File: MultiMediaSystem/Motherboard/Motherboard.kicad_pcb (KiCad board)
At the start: 4 copper layers, 172.8 x 157.7 mm, 43 parts, among them J1 Wire Harness, J10 RF_EN, J14 5V_1, J15 RPI_Buck, J16 AUSB2-4599, J17 Illum/Dim, J18 5V_2, J19 GP_Buck, J2 Vmem Jumper, J20 5V_3, J21 Motherboard bracket, J22 Motherboard bracket, J3 Vacc_jumper, J4 RF_RX, J5 RF_CTRL, J6 AntennaExternal, J7 PwrCtrl_in, J8 RF_TX, J9 AntennaPwr_Conn, K1 ADW1112HTW, Q1 T2N7002BK,LM, U1 AudioAmp_PS, U2 AudioAmp, U3 PowerSupplyCtrl, U4 RadioRegulator, U5 HMC784AMS8GETR, U6 RadioAmp, U7 SN74LVC2G06QDCKRQ1

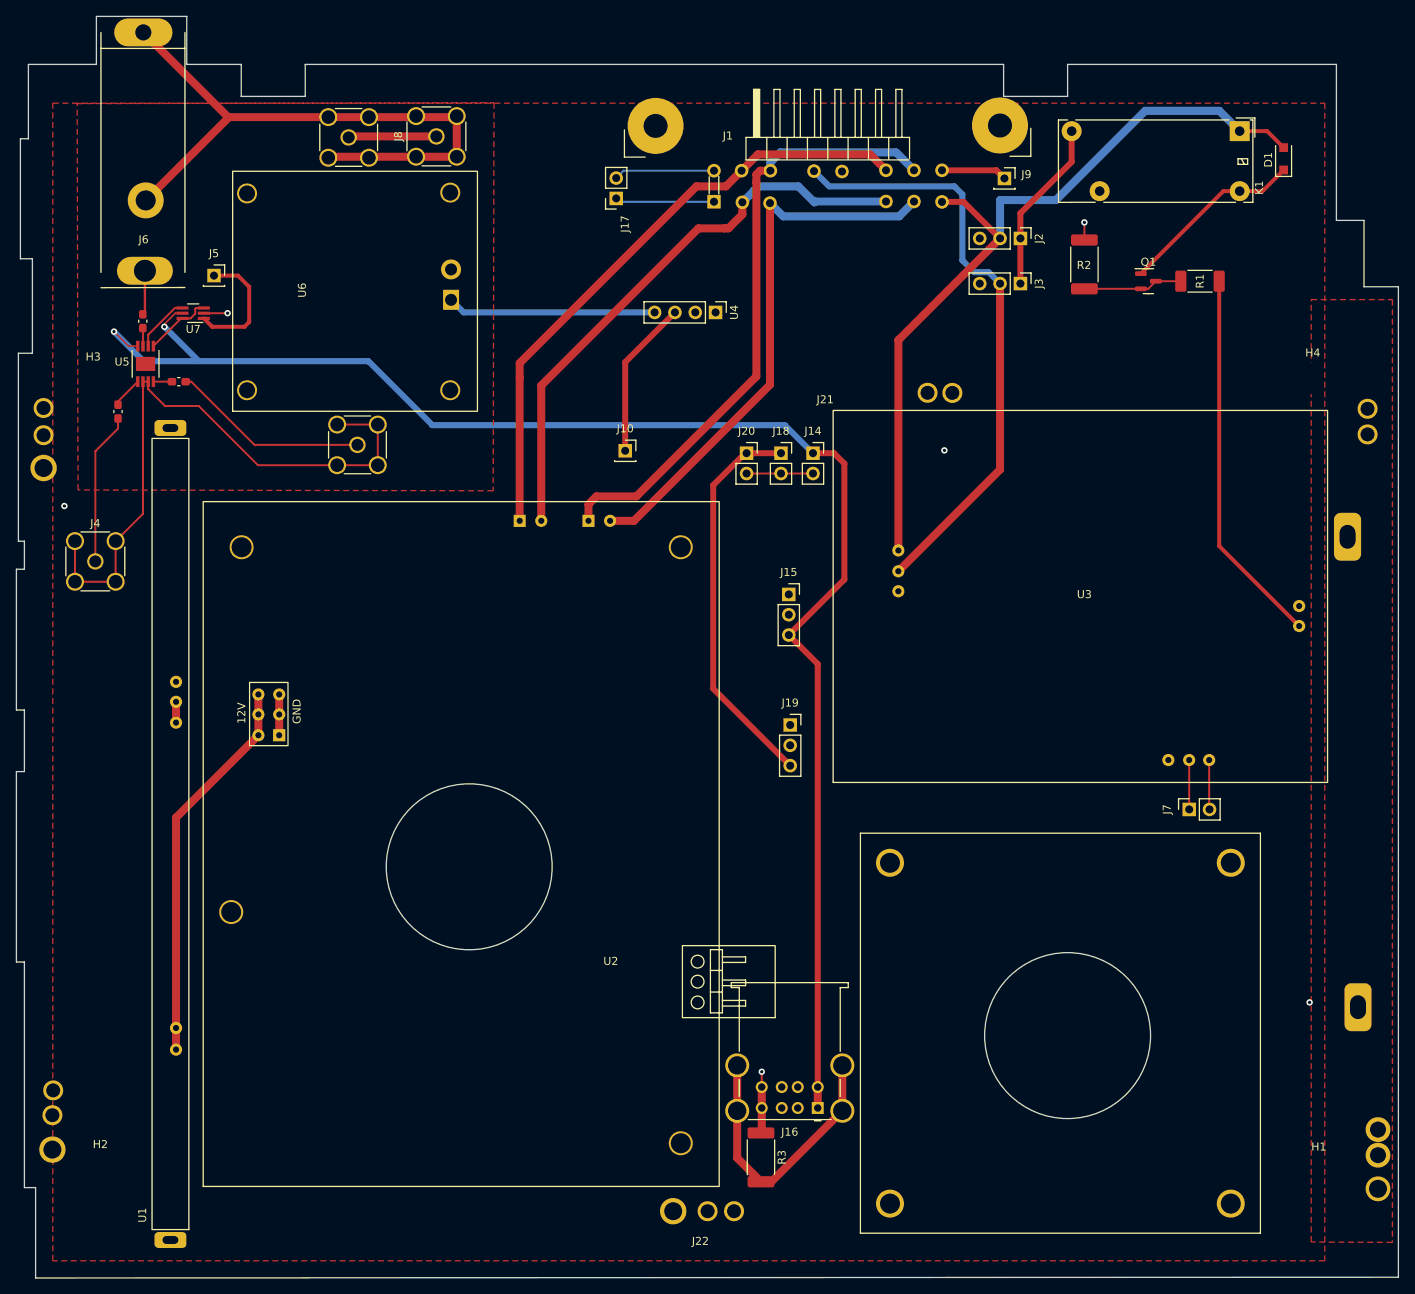
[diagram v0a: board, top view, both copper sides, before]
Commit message: Updated all designs
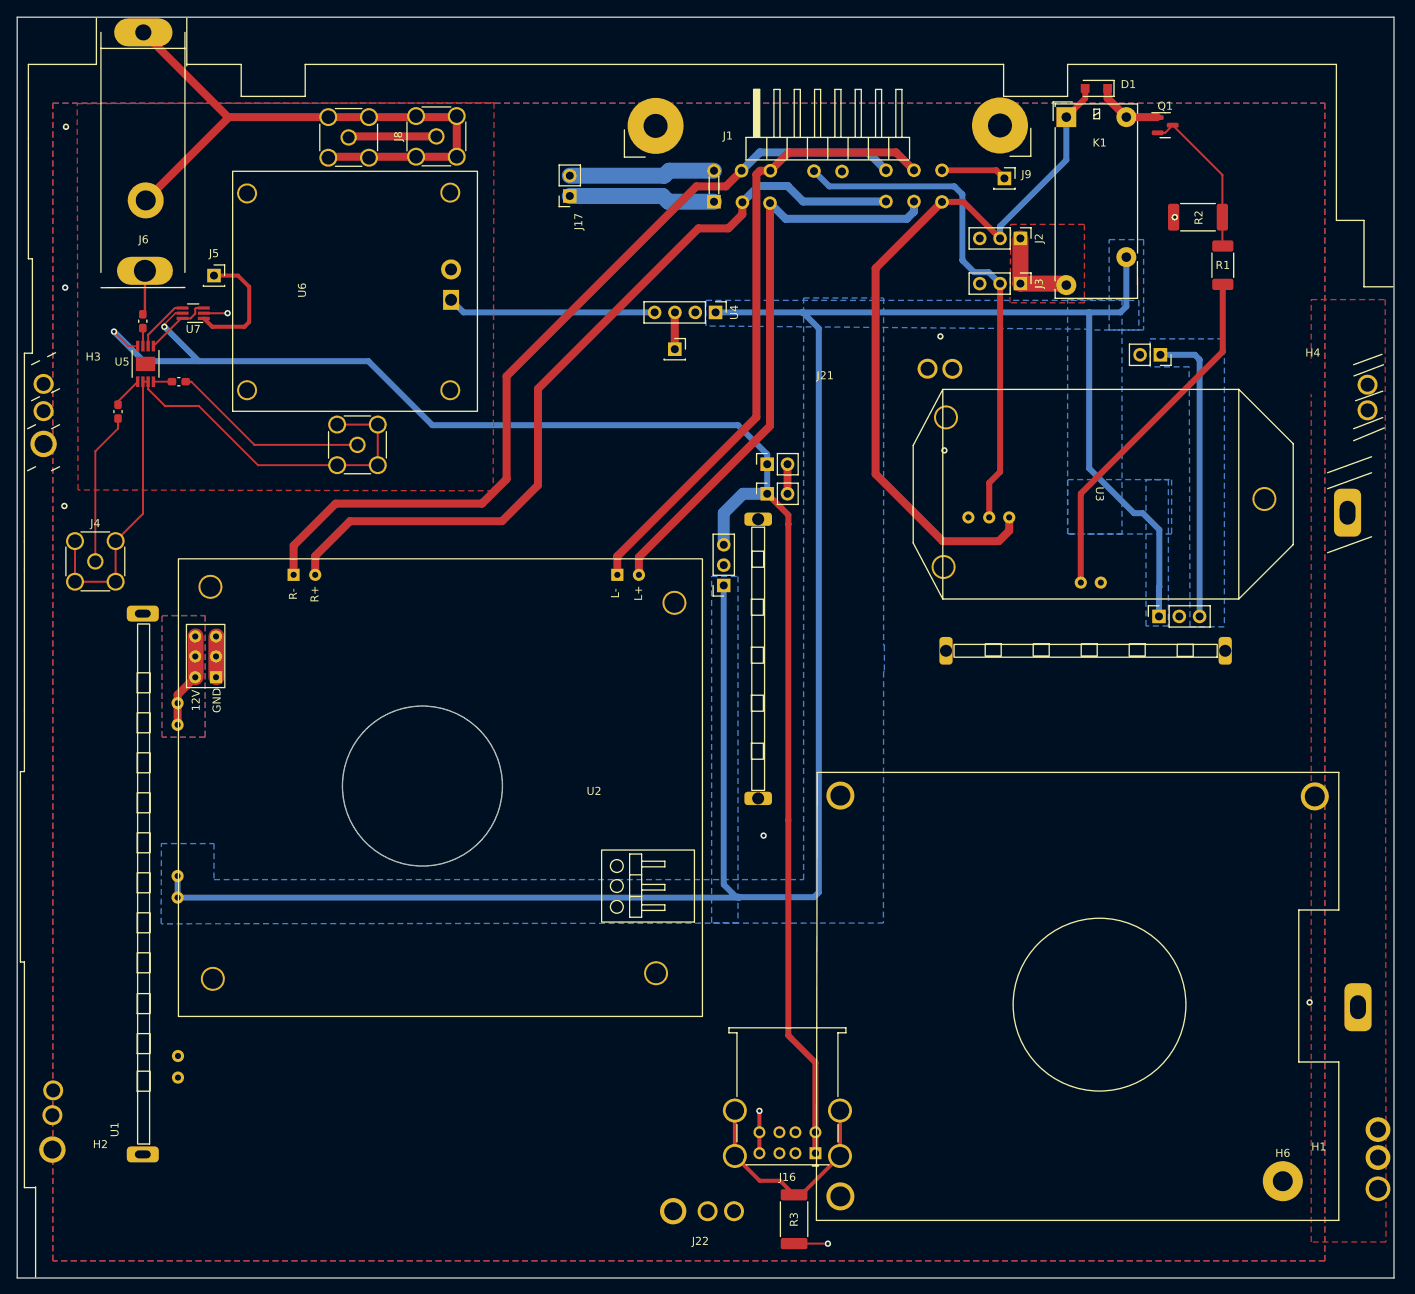
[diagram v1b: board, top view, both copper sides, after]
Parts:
- removed J7: PwrCtrl_in, Connector_PinSocket_2.54mm:PinSocket_1x02_P2.54mm_Vertical
- J15, J19: footprint Connector_PinSocket_2.54mm:PinSocket_1x03_P2.54mm_Vertical -> Custom:5V_Reg_Footprint_VertMnt
- moved J15 54.1 mm to (274.6, 131.1), turned to 90 degrees
- moved U3 50.4 mm to (236.3, 97.3), turned to -90 degrees
- moved J14 45.1 mm to (267.5, 93.3), turned to -90 degrees
- moved D1 25.0 mm to (259.5, 60.0), turned to 180 degrees
- moved J19 24.9 mm to (218.0, 114.8), turned to 180 degrees
- moved K1 21.7 mm to (255.7, 63.6), turned to 0 degrees
- moved U2 21.4 mm to (210.3, 176.0)
- moved Q1 19.6 mm to (268.1, 64.6)
- moved R2 15.4 mm to (272.2, 76.1), turned to 0 degrees
- moved J10 14.1 mm to (206.8, 92.6)
- moved H7 13.4 mm to (286.8, 148.5)
- moved U1 11.2 mm to (142.6, 192.2)
- moved H5 10.4 mm to (227.5, 148.4)
- moved R3 8.77 mm to (221.7, 201.3), turned to 90 degrees
- moved H6 7.08 mm to (282.8, 196.6)
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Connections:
- J16 pad 1: 5V -> 5V_GP
- J16 pad 5: 5V -> 5V_GP
- U5 pad 4: 5V -> 5V_GP
- U7 pad 5: 5V -> 5V_GP
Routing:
- net Vsrc: track 2.60 -> 296.7 mm
- net 5V: track 196.0 -> 37.2 mm, vias 2 -> 0
- net 5V_GP: track 49.2 -> 201.2 mm, vias 0 -> 2
- net AudioPwr: track 48.7 -> 12.0 mm
- net FrontSpkr_R+: track 72.1 -> 101.6 mm
- net FrontSpkr_R-: track 77.1 -> 106.5 mm
- net Radio_EN: track 19.9 -> 4.61 mm
- net Net-(D1-Pad1): track 23.2 -> 8.51 mm
- net Vacc: track 75.1 -> 63.7 mm
- net Vdd: track 21.7 -> 11.5 mm
- net Vmem: track 100.2 -> 92.2 mm
- net Net-(Q1-Pad2): track 12.4 -> 20.0 mm
- net Net-(J16-Pad9): track 35.3 -> 28.5 mm
- net UART_TX: track 6.19 -> 0.00 mm
- net UART_RX: track 6.17 -> 0.00 mm
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- added copper zone on B.Cu, net 5V
- added copper zone on B.Cu, net AudioPwr
- added copper zone on F.Cu, net AudioPwr
- added copper zone on B.Cu, net GND
- added copper zone on F.Cu, net Vdd
- added copper zone on B.Cu, net Vsrc
- removed copper zone on In1.Cu, net GND
- removed copper zone on In2.Cu, net Vsrc
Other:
- board size 172.8 x 157.7 mm -> 172.1 x 157.6 mm
- copper layers 4 -> 2
- board text removed: "MountingHole Error: Too far away from right wall"
